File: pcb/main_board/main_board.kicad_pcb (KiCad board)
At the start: 2 copper layers, 123.7 x 102.1 mm, 42 parts

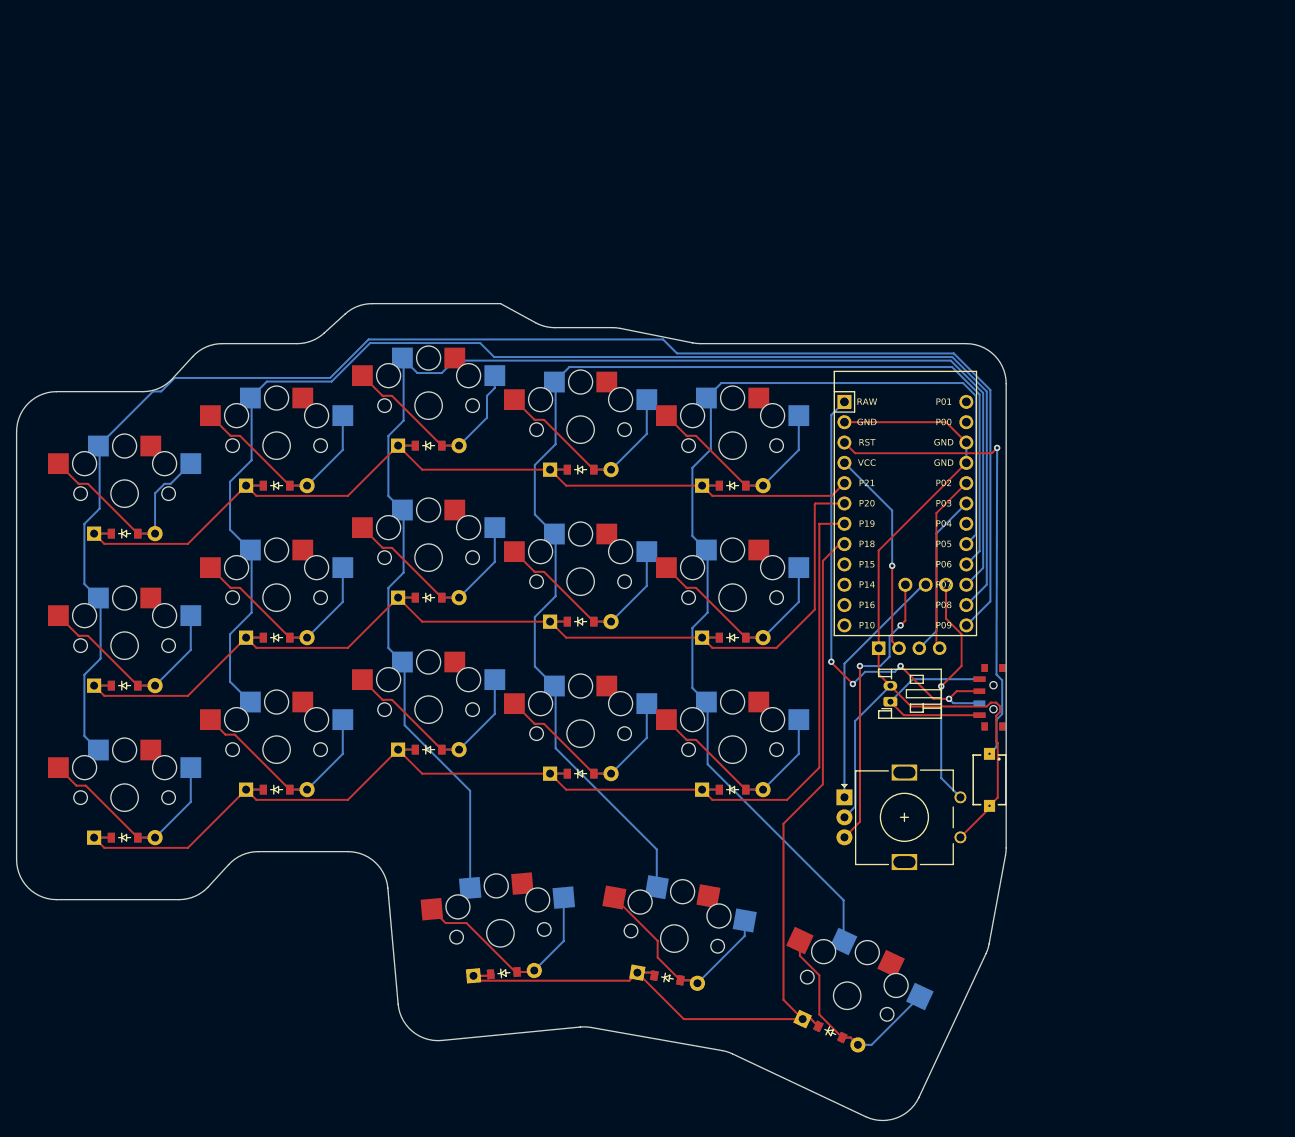
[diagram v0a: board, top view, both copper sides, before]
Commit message: board design 1.0 done
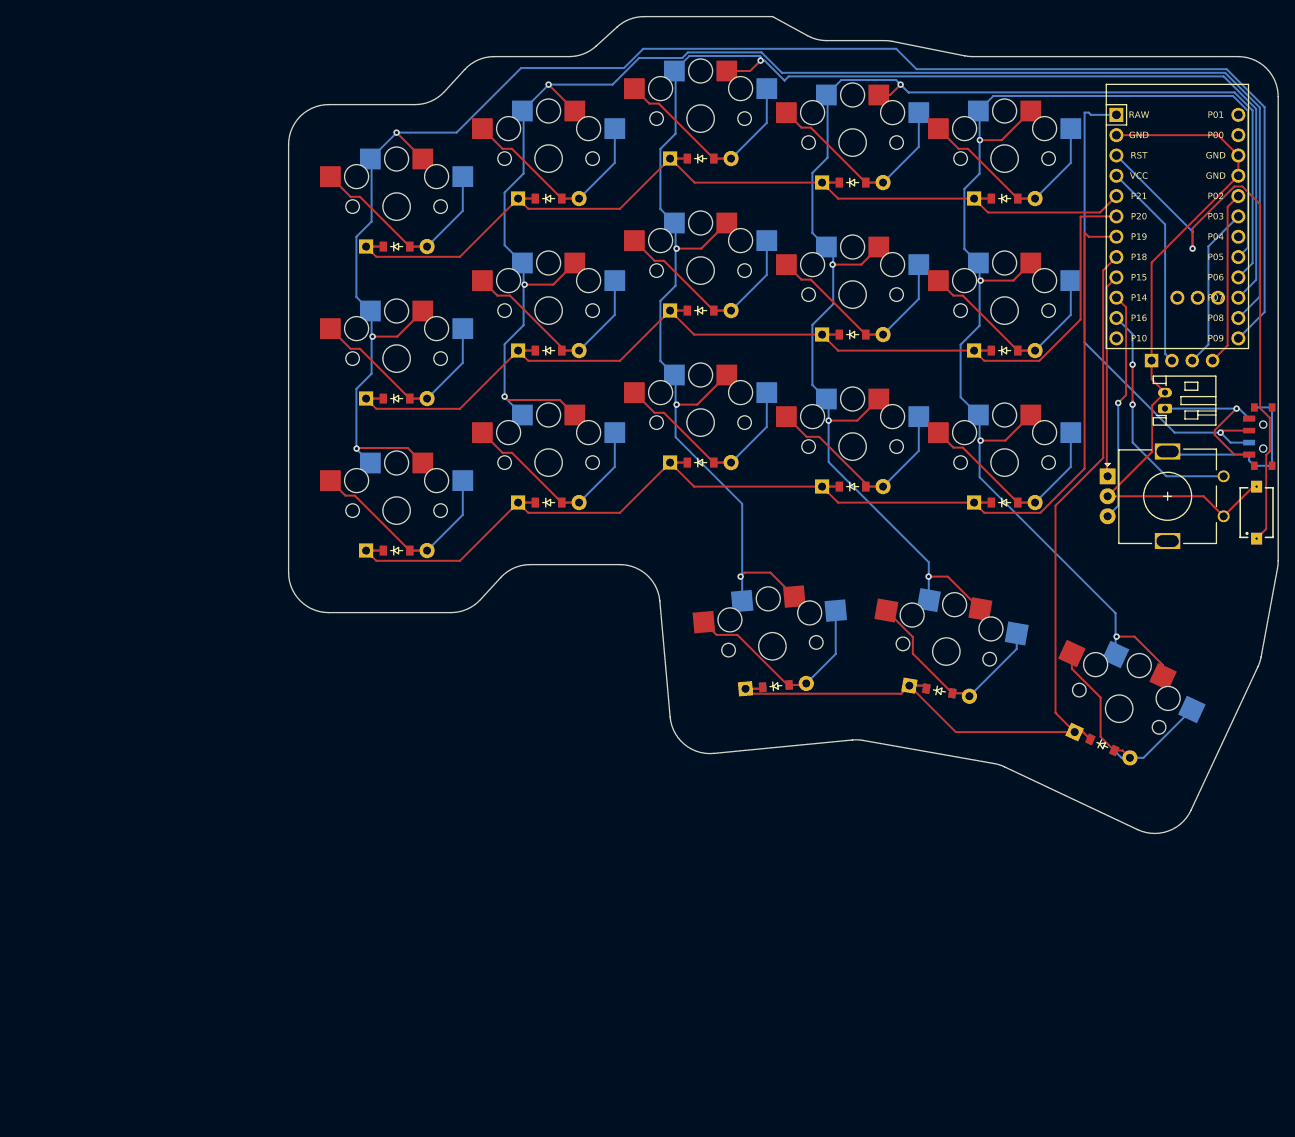
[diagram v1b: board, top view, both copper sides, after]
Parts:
- moved ROT1 51.9 mm to (287.5, 85.5)
- moved _1 50.2 mm to (287.1, 74.5)
- moved OLED1 49.6 mm to (295.2, 66.9)
- moved MCU1 49.4 mm to (288.6, 51.8)
- moved S16 49.4 mm to (238.0, 104.2)
- moved D1 49.4 mm to (191.0, 92.2)
- moved D10 49.4 mm to (248.0, 84.2)
- moved D11 49.4 mm to (248.0, 65.2)
- moved D12 49.4 mm to (248.0, 46.2)
- moved D13 49.4 mm to (267.0, 86.2)
- moved D14 49.4 mm to (267.0, 67.2)
- moved D15 49.4 mm to (267.0, 48.2)
- moved D16 49.4 mm to (238.4, 109.2)
- moved D18 49.4 mm to (279.2, 116.5)
- moved D2 49.4 mm to (191.0, 73.2)
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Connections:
- ROT1 pad 1: NN_101 -> P16
- ROT1 pad A: NN_102 -> P15
- ROT1 pad B: NN_107 -> P14
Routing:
- net NN_107: track 36.2 -> 0.00 mm, vias 2 -> 0
- net P5: track 132.7 -> 164.3 mm, vias 0 -> 4
- net NN_102: track 31.0 -> 0.00 mm
- net P7: track 173.5 -> 203.1 mm, vias 0 -> 4
- net P16: track 0.00 -> 29.5 mm, vias 0 -> 2
- net NN_101: track 29.4 -> 0.00 mm, vias 1 -> 0
- net P14: track 0.00 -> 28.8 mm, vias 0 -> 1
- net P15: track 0.00 -> 25.4 mm
- net P6: track 150.0 -> 175.0 mm, vias 0 -> 4
- net (no net): track 0.00 -> 23.7 mm
- net P9: track 191.6 -> 213.4 mm, vias 0 -> 3
- net P8: track 167.6 -> 189.3 mm, vias 0 -> 3
- net GND: track 104.4 -> 88.2 mm
- net RST: track 59.2 -> 72.6 mm
- net pos: track 24.1 -> 20.8 mm, vias 0 -> 1
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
